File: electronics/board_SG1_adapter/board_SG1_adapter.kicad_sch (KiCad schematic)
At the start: 21 parts, among them J1 Conn_01x01, J2 Conn_01x01, J3 Conn_01x03, J4 Conn_01x03, T1 10P_1P_2S

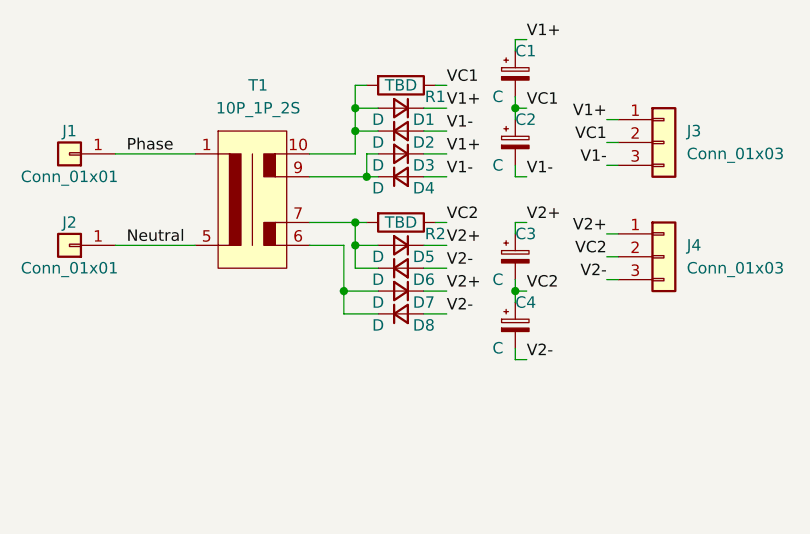
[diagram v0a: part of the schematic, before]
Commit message: WIP rectifier section
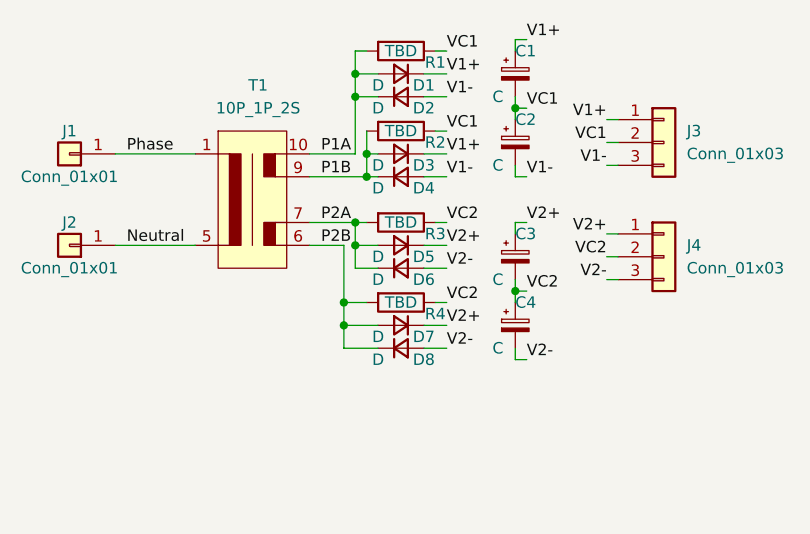
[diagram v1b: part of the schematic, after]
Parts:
- added R3, R4: TBD, SquantorRcl:R_1206, symbol Device:R
- D1, D2, D3, D4, D5, D6, D7, D8: footprint Diode_SMD:D_SMA -> Diode_SMD:D_SMB
- T1: footprint (none) -> SquantorTransformer:10pin_5pitch_32x27_1Pri_2Sec
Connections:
- net VC1: now also R2.1
- net VC2: now also R3.1, R4.1; no longer R2.1
- net P1B: now reaches D3.2 (A), D4.1 (K), T1.9
- net P1B: now also R2.2
- net P2A: now reaches D5.2 (A), D6.1 (K), T1.7
- net P2A: now also R3.2; no longer R2.2
- net P1A: now reaches D1.2 (A), D2.1 (K), R1.2, T1.10
- net P2B: now reaches D7.2 (A), D8.1 (K), T1.6
- net P2B: now also R4.2
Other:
- moved on the sheet: D1, D2, D7, D8, R1, R2
